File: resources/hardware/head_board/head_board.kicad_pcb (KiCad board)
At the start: 2 copper layers, 66 x 61 mm, 23 parts, among them IC1 ATMEGA328P-P, P1 SERIAL, P2 PI_CONN, P3 REED, P4 PR, P5 CAM_LEDS, P6 STEPPER, P7 PR_LED, P8 FDBK_LED, Q1 BC547, Q2 BC547

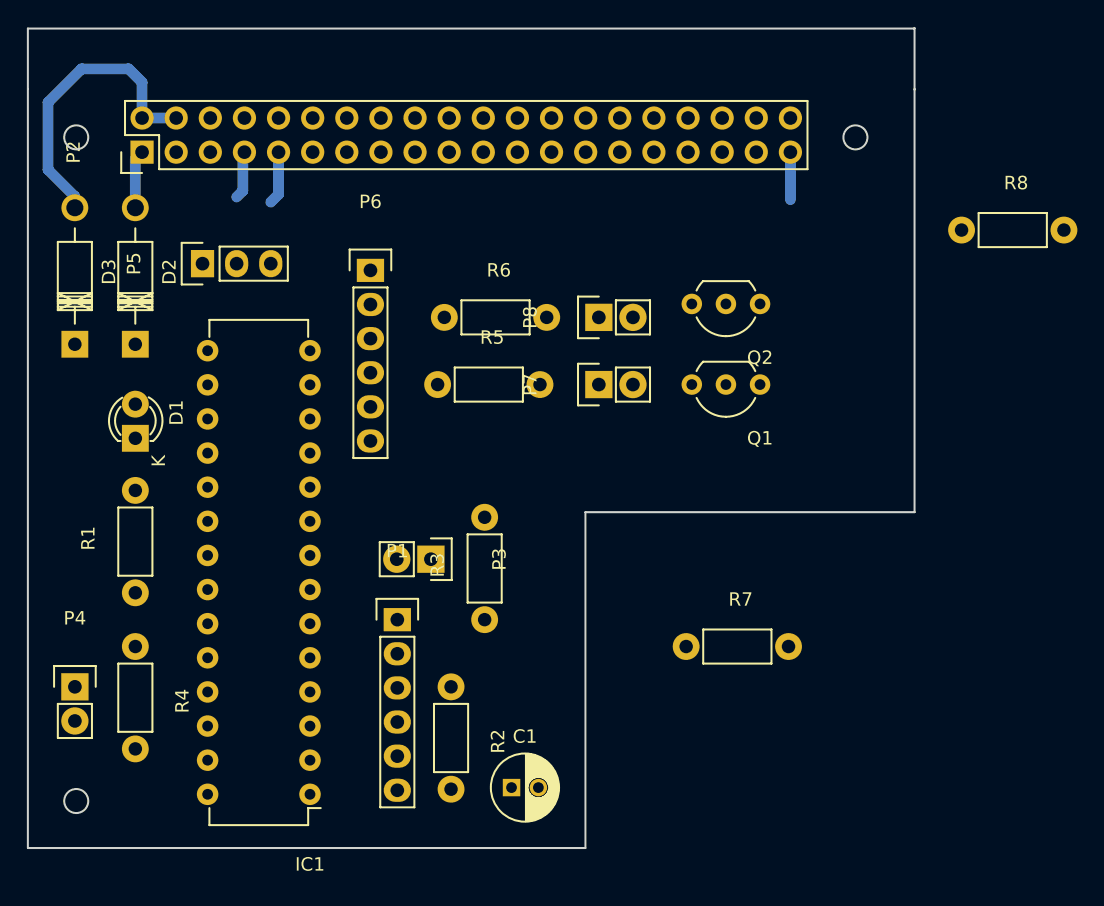
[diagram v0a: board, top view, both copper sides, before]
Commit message: finished new headboard pcbs
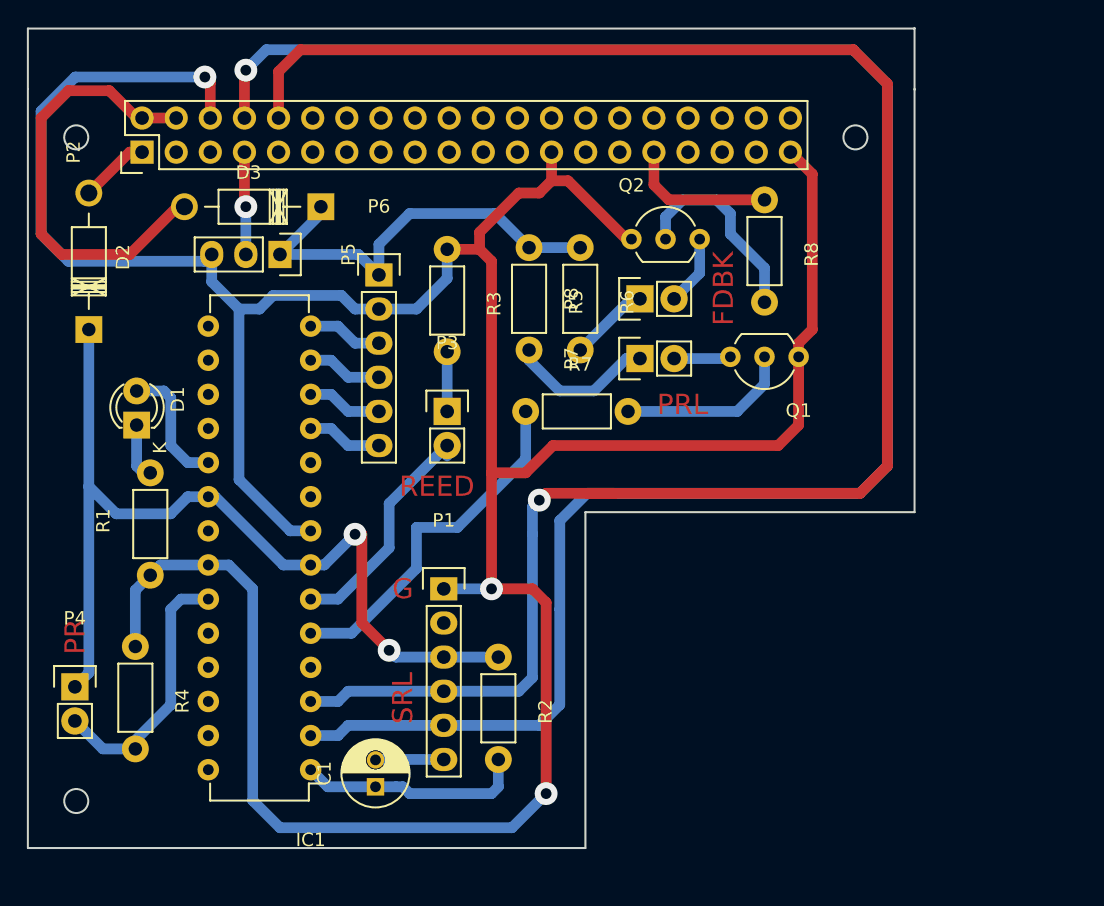
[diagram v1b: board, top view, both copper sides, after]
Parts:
- moved R3 27.7 mm to (156.2, 114.9), turned to 270 degrees
- moved R7 21.2 mm to (162.1, 127.0)
- moved D3 21.0 mm to (146.8, 111.8), turned to 180 degrees
- moved R8 14.8 mm to (179.8, 111.3), turned to 270 degrees
- moved R5 12.3 mm to (162.3, 114.8), turned to 270 degrees
- moved R6 11.4 mm to (166.1, 114.8), turned to 270 degrees
- moved P3 11.1 mm to (156.2, 127.0), turned to 0 degrees
- moved Q2 10.7 mm to (169.9, 114.2), turned to 0 degrees
- moved C1 10.1 mm to (150.9, 154.9), turned to 90 degrees
- moved P5 5.80 mm to (143.8, 115.3), turned to 270 degrees
- moved R2 4.16 mm to (160.0, 145.3)
- moved P1 4.15 mm to (156.0, 140.2)
- moved D2 3.63 mm to (129.5, 120.9)
- moved P7 3.62 mm to (170.6, 123.1)
- moved Q1 3.54 mm to (182.4, 122.9)
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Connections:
- P2 pad 17: +3V3 -> (no net)
- P2 pad 18: /FDBK -> (no net)
- P2 pad 31: (no net) -> /FDBK
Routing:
- net GND: track 7.50 -> 251.4 mm, vias 0 -> 3
- net /PITX: track 0.00 -> 140.8 mm, vias 0 -> 1
- net /PIRX: track 0.00 -> 138.6 mm, vias 0 -> 1
- net +3V3: track 0.00 -> 69.6 mm, vias 0 -> 2
- net /PRLED: track 0.00 -> 39.7 mm
- net +5V: track 0.00 -> 32.1 mm
- net /PR: track 0.00 -> 20.0 mm
- net /REED: track 0.00 -> 17.6 mm
- net /RST: track 0.00 -> 16.9 mm
- net Net-(Q2-Pad2): track 0.00 -> 15.1 mm
- net /FDBK: track 0.00 -> 11.1 mm
- net Net-(P7-Pad1): track 0.00 -> 11.0 mm
- net Net-(D3-Pad2): track 22.3 -> 33.1 mm
- net /LED: track 0.00 -> 9.63 mm
- net Net-(P8-Pad1): track 0.00 -> 6.02 mm
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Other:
- net class Default: via_dia 1.4 -> 1.7
- board text added: "FDBK"
- board text added: "G"
- board text added: "PR"
- board text added: "PRL"
- board text added: "REED"
- board text added: "SRL"
